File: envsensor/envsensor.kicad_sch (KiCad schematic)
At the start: 6 parts, among them U1 LD2450, U3 SCD30, U4 MS5611-01BA, U5 BH1750, U6 ZJY_M150_128x128_7P

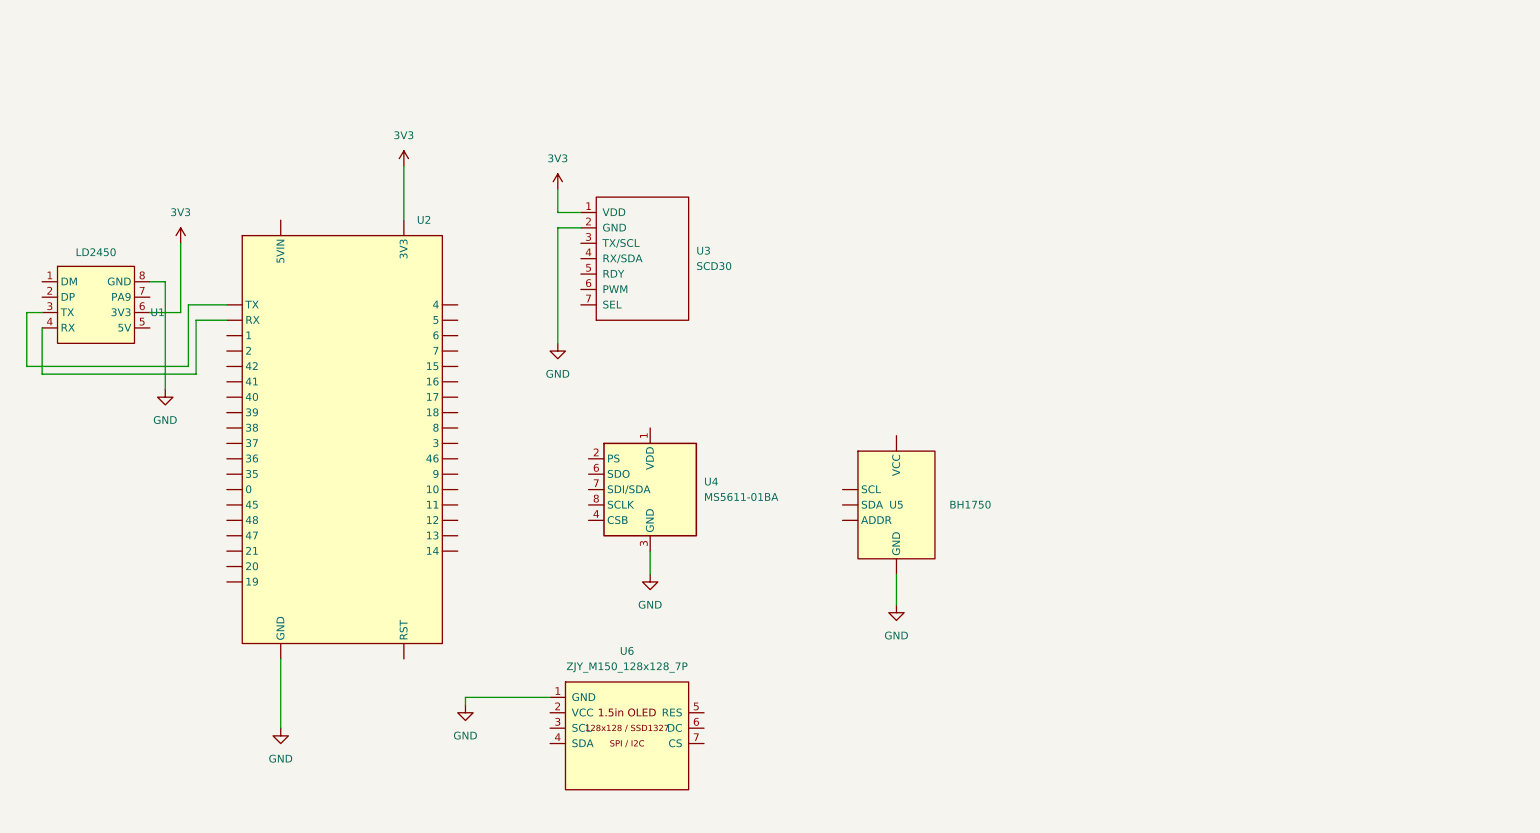
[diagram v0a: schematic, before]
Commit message: final version
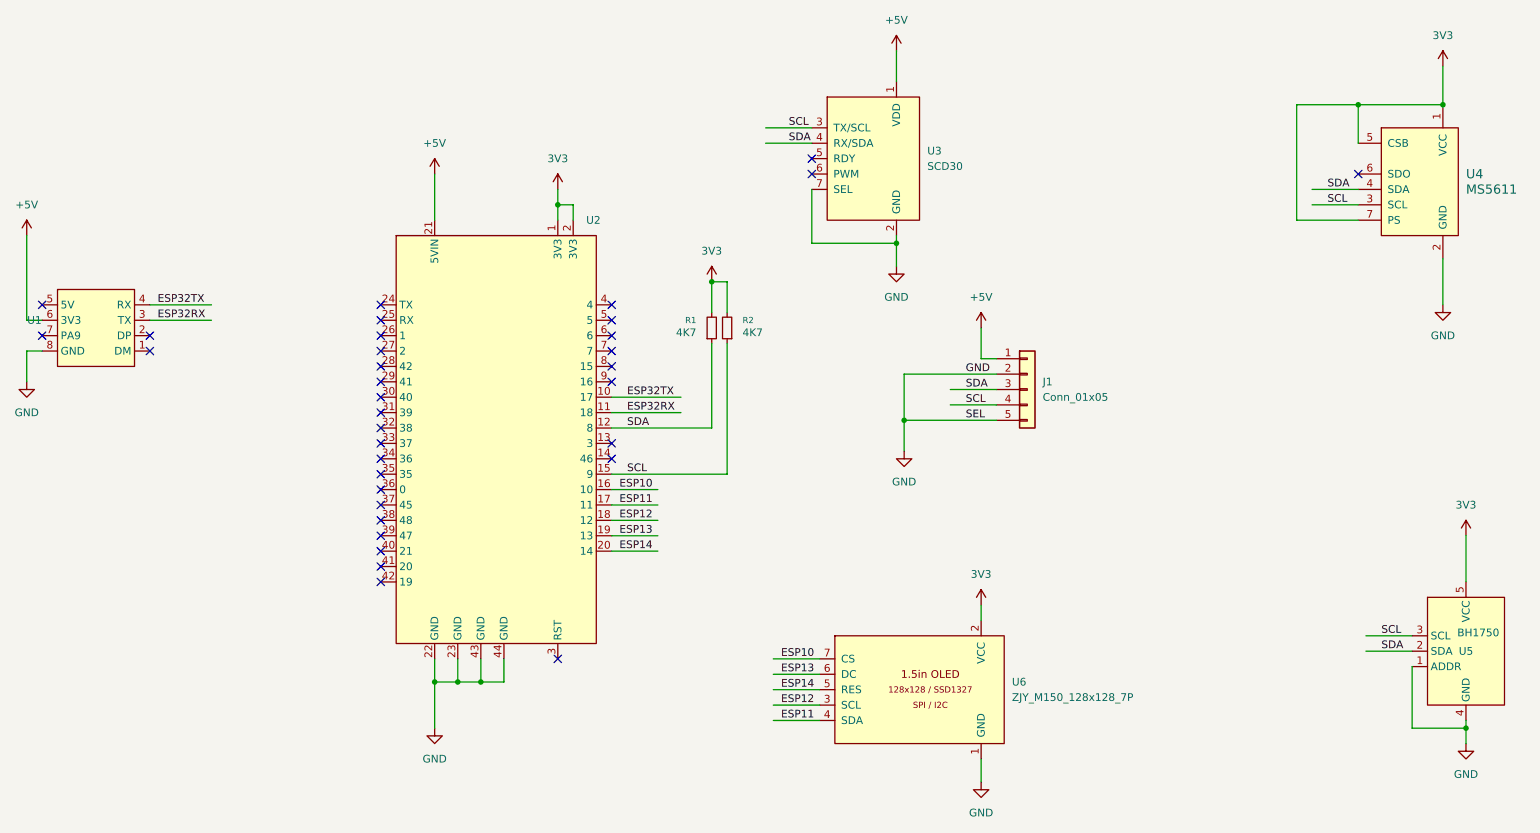
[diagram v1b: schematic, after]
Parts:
- removed U6: ZJY_M150_128x128_7P, ZJY_M150_128x128_7P:ZJY_M150_128x128_7P, symbol SSD1327_ZJY_M150:ZJY_M150_128x128_7P
- added J1: Conn_01x05, Connector_PinHeader_2.54mm:PinHeader_1x05_P2.54mm_Vertical, symbol Connector_Generic:Conn_01x05
- added R1, R2: 4K7, Resistor_SMD:R_0603_1608Metric, symbol Device:R_Small
- added U6: ZJY_M150_128x128_7P, Library:ZJY_M150_128x128_7P, symbol New_Library:ZJY_M150_128x128_7P
- U1: value LD2450 -> (none)
- U4: value MS5611-01BA -> MS5611; footprint Package_LGA:LGA-8_3x5mm_P1.25mm -> (none); symbol Sensor_Pressure:MS5611-01BA -> New_Library:MS5611
- U5: symbol bh1750:_1 -> New_Library:BH1750
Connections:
- net 3V3: now also U2.1 (3V3), U2.2 (3V3), U4.1 (VCC), U4.5 (CSB), U4.7 (PS), U5.5 (VCC), R1.2, R2.2, U6.2 (VCC); no longer U1.6 (3V3), U2. (14), U3.1 (VDD)
- net GND: now also U2.22 (GND), U2.23 (GND), U2.43 (GND), U2.44 (GND), U3.7 (SEL), U4.2 (GND), U5.1 (ADDR), U5.4 (GND), J1.2 (Pin_2), J1.5 (Pin_5), U6.1 (GND); no longer U2. (14), U4.3 (GND), U5. (GND)
- net ESP32RX: now reaches U1.3 (TX)
- net ESP32RX: now also U2.11 (18); no longer U2. (14)
- net ESP32TX: now reaches U1.4 (RX)
- net ESP32TX: now also U2.10 (17); no longer U2. (14)
- net SDA: now reaches U4.4 (SDA)
- net SDA: now also U2.12 (8), U3.4 (RX/SDA), U5.2 (SDA), J1.3 (Pin_3), R1.1; no longer U4.5 (CSB)
- net SCL: now reaches U3.3 (TX/SCL)
- net SCL: now also U2.15 (9), U4.3 (SCL), U5.3 (SCL), J1.4 (Pin_4), R2.1
- new net +5V: J1.1 (Pin_1), U1.6 (3V3), U2.21 (5VIN), U3.1 (VDD)
- new net ESP10: U2.16 (10), U6.7 (CS)
- new net ESP11: U2.17 (11), U6.4 (SDA)
- new net ESP12: U2.18 (12), U6.3 (SCL)
- new net ESP13: U2.19 (13), U6.6 (DC)
- new net ESP14: U2.20 (14), U6.5 (RES)
- no-connect marks 0 -> 35
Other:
- moved on the sheet: U1, U4
